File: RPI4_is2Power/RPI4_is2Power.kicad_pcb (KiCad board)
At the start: 4 copper layers, 65 x 56 mm, 27 parts, among them J1 GPIO, J11 5v pin, J2 Conn_01x03_Socket, J3 U.FL-R-SMT-1_80_, J4 U.FL-R-SMT-1_80_, J5 U.FL-R-SMT-1_80_, J6 U.FL-R-SMT-1_80_, J7 U.FL-R-SMT-1_80_, J8 5v pin, J9 5v pin

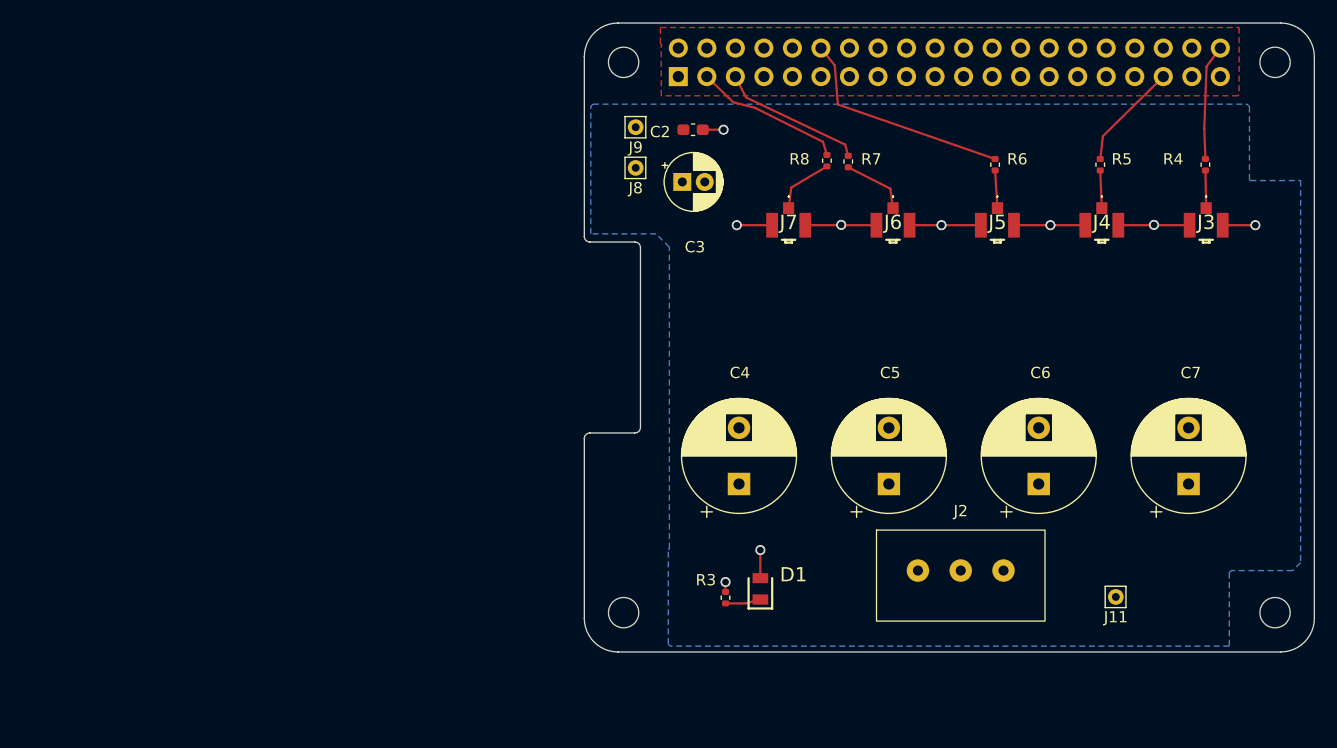
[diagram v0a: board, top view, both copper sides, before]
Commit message: updated final four boards for streamer
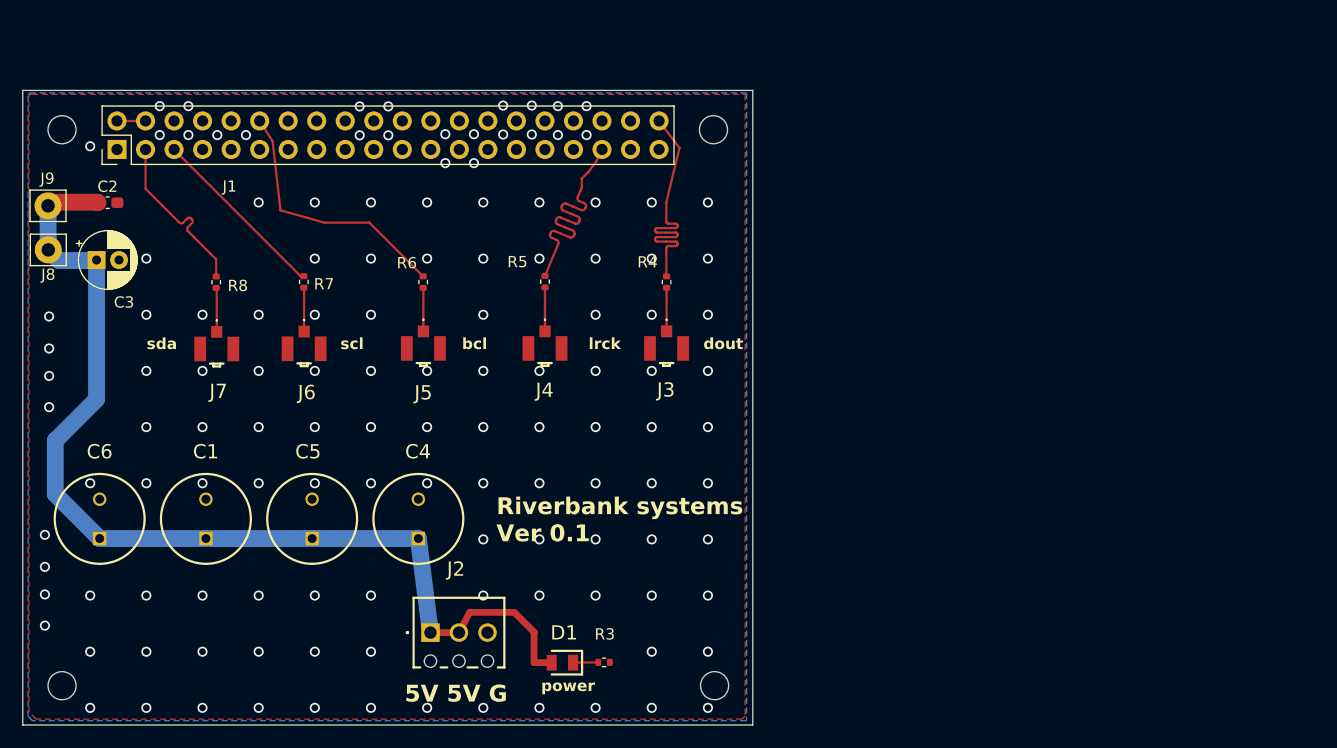
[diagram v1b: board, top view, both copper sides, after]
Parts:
- removed C7: 470u, Capacitor_THT:CP_Radial_D10.0mm_P5.00mm
- removed J11: 5v pin, Connector_Pin:Pin_D0.7mm_L6.5mm_W1.8mm_FlatFork
- removed MH1, MH2, MH3, MH4: MountingHole_2.7mm_M2.5, MountingHole:MountingHole_2.7mm_M2.5
- added C1: 330u, samsys:CAPPRD350W60D800H1300, F.Cu at (66.3, 89.9)
- added H1: MountingHole, MountingHole:MountingHole_2.5mm, F.Cu at (53.5, 53.5)
- added H2: MountingHole, MountingHole:MountingHole_2.5mm, F.Cu at (111.5, 53.5)
- added H3: MountingHole, MountingHole:MountingHole_2.5mm, F.Cu at (53.5, 103.2)
- added H4: MountingHole, MountingHole:MountingHole_2.5mm, F.Cu at (111.6, 103.0)
- C4, C5, C6: value 470u -> 330u; footprint Capacitor_THT:CP_Radial_D10.0mm_P5.00mm -> samsys:CAPPRD350W60D800H1300
- J1: moved to F.Cu
- J2: value Conn_01x03_Socket -> 1725669; footprint samsys:PCB Wired Socket -> samsys:1725669
- J8, J9: value 5v pin -> Conn_01x01_Pin; footprint Connector_Pin:Pin_D0.7mm_L6.5mm_W1.8mm_FlatFork -> Connector_Pin:Pin_D1.2mm_L11.3mm_W3.0mm_Flat
- moved C6 83.7 mm to (56.9, 89.9)
- moved R8 55.4 mm to (67.2, 67.1)
- moved J6 53.6 mm to (75.0, 73.0)
- moved J8 52.8 mm to (52.3, 64.2)
- moved J9 52.8 mm to (52.2, 60.3)
- moved C3 52.6 mm to (56.6, 65.1)
- moved C2 52.5 mm to (57.6, 60.0)
- moved J5 52.3 mm to (85.7, 73.0)
- moved J7 52.1 mm to (67.3, 73.0)
- moved R6 52.0 mm to (85.7, 67.1)
- moved C5 51.6 mm to (75.8, 89.9)
- moved J4 50.8 mm to (96.5, 73.0)
- moved R5 50.5 mm to (96.5, 67.0)
- moved J1 50.1 mm to (58.4, 52.7), turned to 90 degrees
- moved R7 49.6 mm to (75.0, 67.0)
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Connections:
- J1 pad 2: Net-(J1-Pin_2) -> unconnected-(J1-Pin_2-Pad2)
- J1 pad 4: Net-(J1-Pin_2) -> unconnected-(J1-Pin_2-Pad2)
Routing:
- net +5V: track 2.50 -> 93.4 mm, vias 1 -> 0
- net GND: track 34.2 -> 0.00 mm, vias 8 -> 128
- net /GPIO21/I2S DOUT: track 10.3 -> 23.7 mm
- net /GPIO19/I2S LRCK: track 9.60 -> 22.7 mm
- net /GPIO3/SCL1: track 12.9 -> 16.2 mm
- net /GPIO18/I2S BCL: track 20.3 -> 23.2 mm
- net unconnected-(J1-Pin_2-Pad2): track 0.00 -> 2.54 mm
- net /GPIO2/SDA1: track 13.3 -> 15.5 mm
- net Net-(J6-SIG): track 5.95 -> 3.93 mm
- net Net-(J7-SIG): track 5.53 -> 3.94 mm
- net Net-(D1-K): track 3.15 -> 2.25 mm
- net Net-(J4-SIG): track 3.35 -> 3.95 mm
- net Net-(J5-SIG): track 3.36 -> 3.94 mm
- net Net-(J3-SIG): track 3.35 -> 3.88 mm
- added copper zone on B.Cu, net GND
- removed copper zone on In2.Cu, net +5V
- removed copper zone on In1.Cu, net GND
- removed copper zone on B.Cu, net GND2
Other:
- board size 65 x 56 mm -> 65 x 56.5 mm
- copper layers 4 -> 2
- board text added: "5V 5V G"
- board text added: "Riverbank systems Ver 0.1"
- board text added: "bcl"
- board text added: "dout"
- board text added: "lrck"
- board text added: "power"
- board text added: "scl"
- board text added: "sda"
- board text removed: "DISPLAY (OPTIONAL)"
- board text removed: "Extend PCB edge 0.5mm if using SMT header"
- board text removed: "PoE"
- board text removed: "RJ45"
- board text removed: "USB"
